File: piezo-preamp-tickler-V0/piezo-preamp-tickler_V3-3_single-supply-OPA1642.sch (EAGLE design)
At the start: 62 parts, among them IC1 OPA1642, Q2 MMBFJ201, SW2-SPST INPUT-select

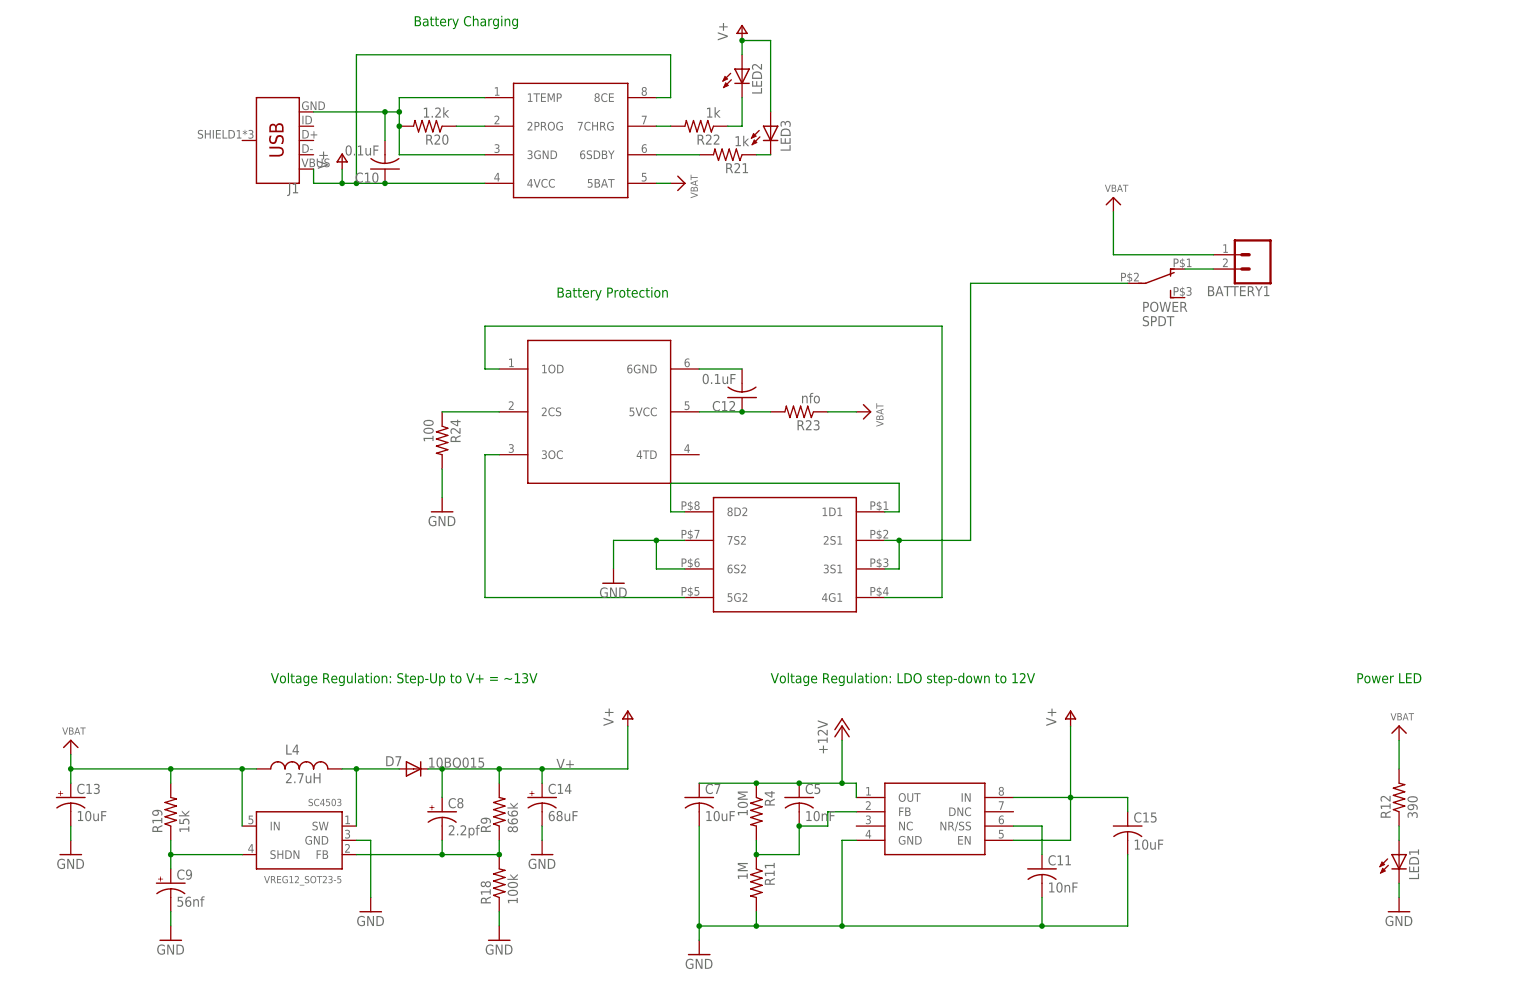
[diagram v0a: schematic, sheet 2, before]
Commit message: piezo preamp updates
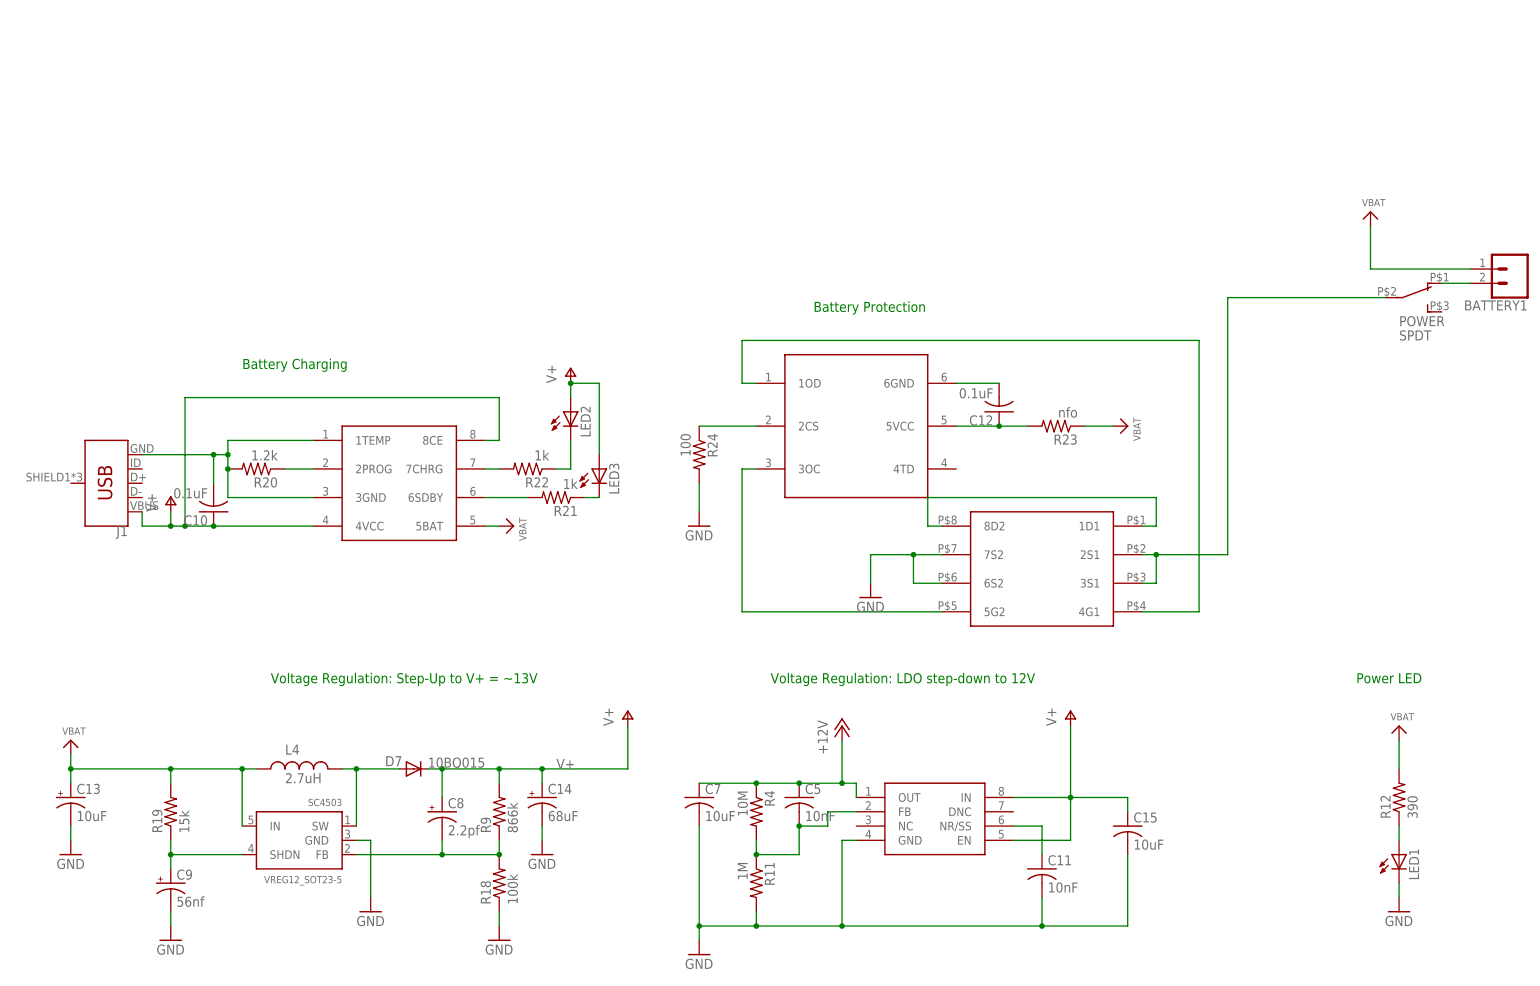
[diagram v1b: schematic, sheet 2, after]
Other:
- moved on the sheet: BATTERY1, C10, C12, J1, LED2, LED3, POWER, R20, R21, R22, R23, R24
